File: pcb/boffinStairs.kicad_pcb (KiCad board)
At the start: 2 copper layers, 17.8 x 19.7 mm, 7 parts, among them P1 CONN_01X05, U1 LM393

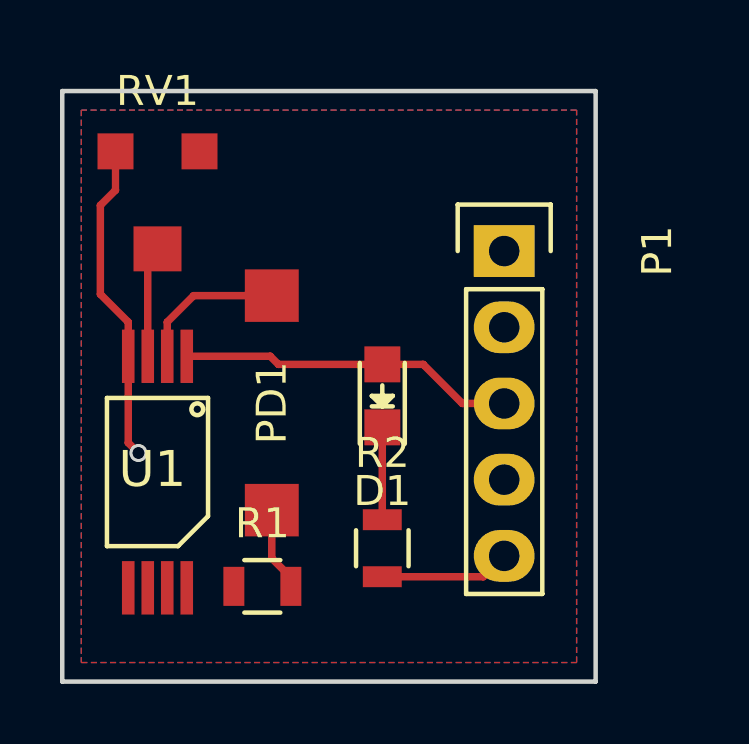
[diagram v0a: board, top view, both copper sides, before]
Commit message: new file:   boffinStairs-B.Cu.gbr 	new file:   boffinStairs-B.SilkS.gbr 	new file:   boffinStairs-Edge.Cuts.gbr 	new file:   boffinStairs-F.Cu.gbr 	new file:   boffinStairs-F.SilkS.gbr 	new file:   boffinStairs-bottom.pos 	new file:   boffinStairs-top.pos 	new file:   boffinStairs.drl 	modified:   boffinStairs.kicad_pcb 	modified:   boffinStairs.kicad_pcb-bak
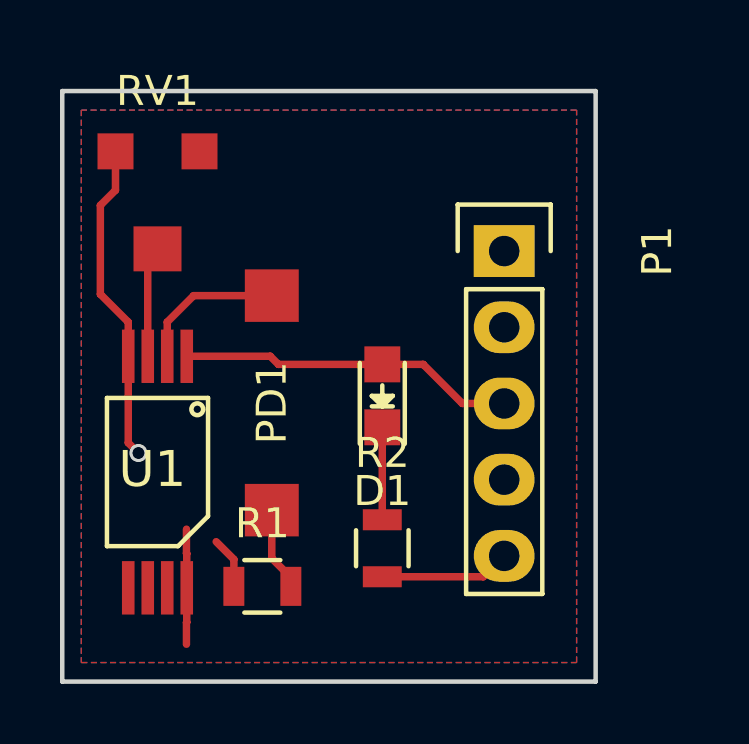
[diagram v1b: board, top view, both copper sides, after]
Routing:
- net VCC: track 0.07 -> 5.65 mm
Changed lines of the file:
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@@
   (general
     (links 14)
-    (no_connects 5)
-    (area 149.784999 97.714999 167.715001 117.550001)
+    (no_connects 1)
+    (area 149.01156 96.665 170.667 117.550001)
     (thickness 1.6)
     (drawings 4)
-    (tracks 26)
+    (tracks 34)
     (zones 0)
     (modules 7)
@@
     (visible_elements FFFFFF7F)
     (pcbplotparams
-      (layerselection 0x00030_80000001)
+      (layerselection 0x01030_80000001)
       (usegerberextensions false)
       (excludeedgelayer true)
@@
       (outputformat 1)
       (mirror false)
-      (drillshape 1)
+      (drillshape 0)
       (scaleselection 1)
       (outputdirectory ""))
@@
   (segment (start 160.02 106.90098) (end 157.06598 106.90098) (width 0.25) (layer F.Cu) (net 1))
   (segment (start 160.528 112.08) (end 160.528 108.99902) (width 0.25) (layer F.Cu) (net 2))
+  (segment (start 155.58 114.3) (end 155.58 113.4) (width 0.25) (layer F.Cu) (net 3))
+  (segment (start 155.58 113.4) (end 154.9908 112.8108) (width 0.25) (layer F.Cu) (net 3))
+  (segment (start 154.0002 115.4998) (end 154.0002 116.2304) (width 0.25) (layer F.Cu) (net 3))
+  (segment (start 154.01 114.35) (end 154.01 115.49) (width 0.25) (layer F.Cu) (net 3))
+  (segment (start 154.01 115.49) (end 154.0002 115.4998) (width 0.25) (layer F.Cu) (net 3))
+  (segment (start 154.0002 113.2002) (end 154.0002 112.395) (width 0.25) (layer F.Cu) (net 3))
+  (segment (start 154.01 114.35) (end 154.01 113.21) (width 0.25) (layer F.Cu) (net 3))
+  (segment (start 154.01 113.21) (end 154.0002 113.2002) (width 0.25) (layer F.Cu) (net 3))
   (segment (start 154.06 114.3) (end 154.01 114.35) (width 0.25) (layer F.Cu) (net 3))
   (segment (start 160.528 113.98) (end 163.896 113.98) (width 0.25) (layer F.Cu) (net 4))
